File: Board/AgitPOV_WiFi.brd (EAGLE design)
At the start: 41.5 x 67.6 mm, 45 parts, among them U1 MMA8452Q

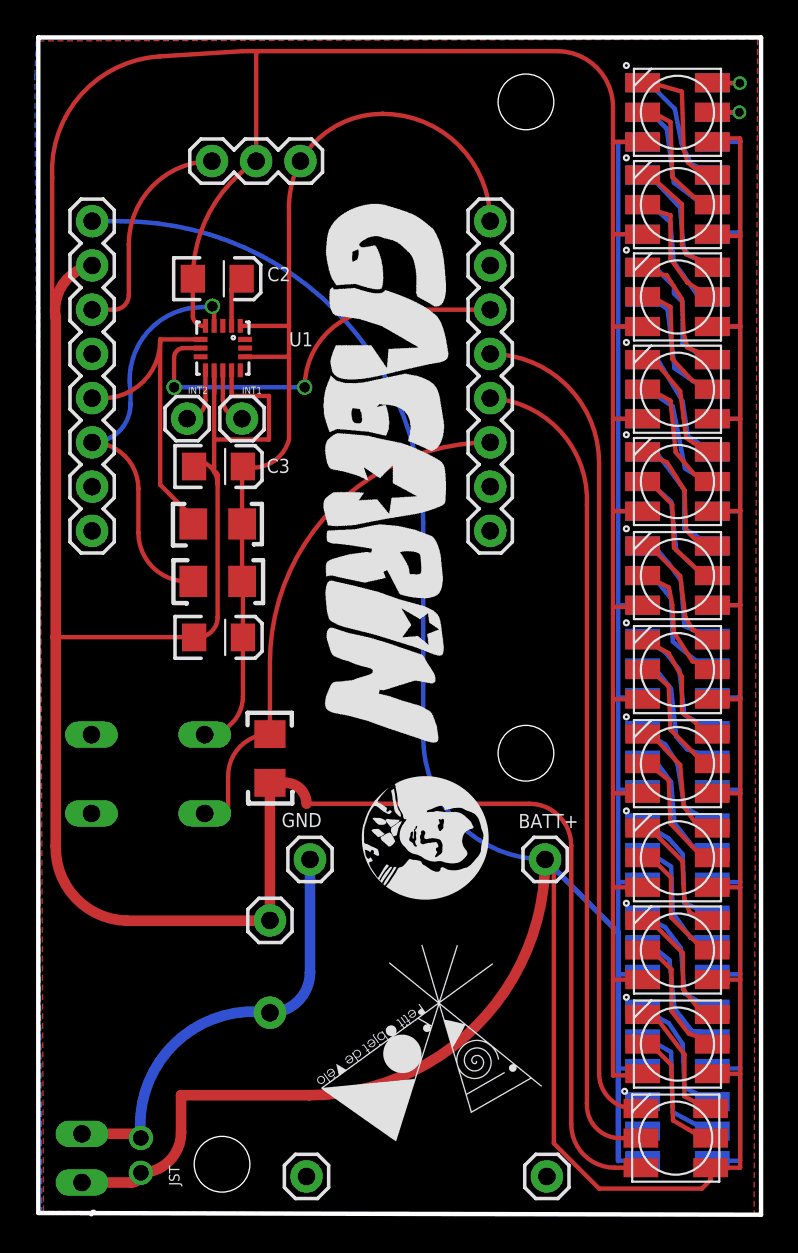
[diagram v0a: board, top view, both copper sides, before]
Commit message: Mean and lean board
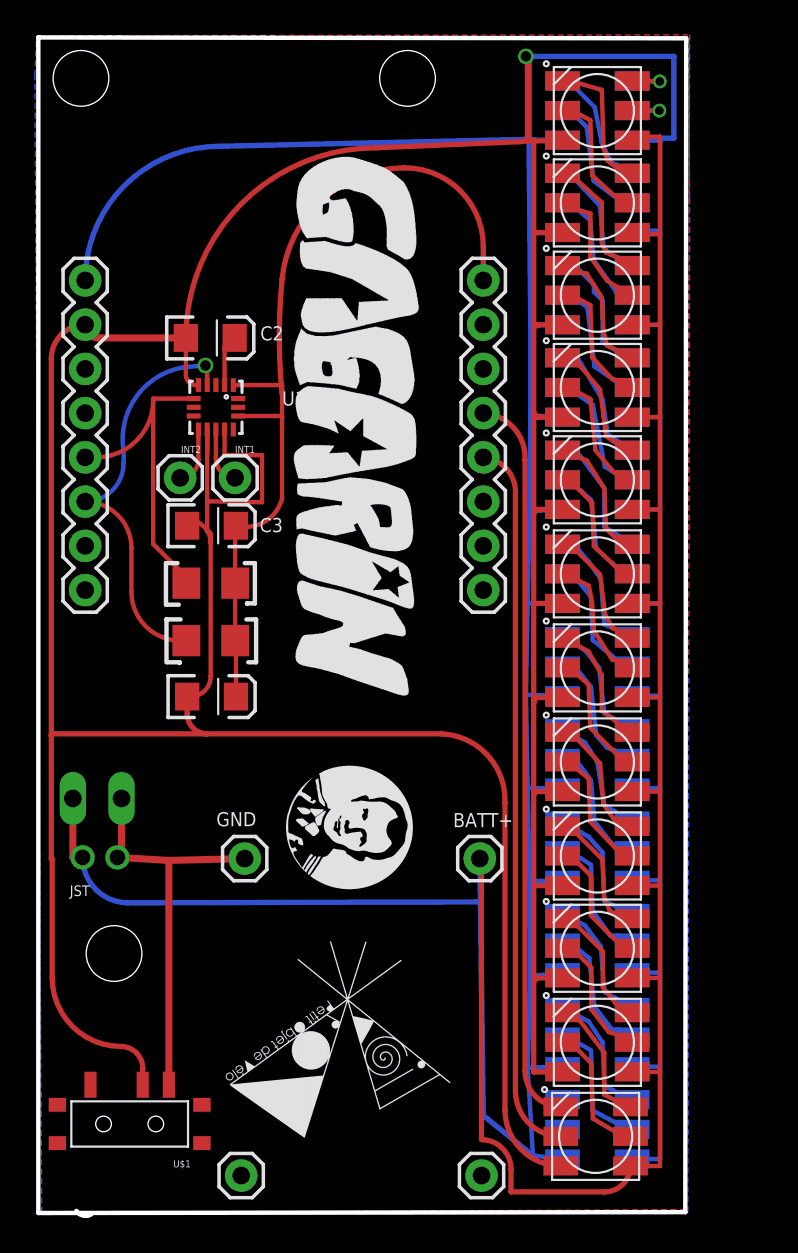
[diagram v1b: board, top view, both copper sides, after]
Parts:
- removed HALL: Hall, SparkFun-Connectors:1X03
- removed JP-GND: SWITCH, SparkFun-Connectors:1X01
- removed JP-GNDE: -, SparkFun-Connectors:1X01
- removed PUSHBUTTON: (no value), switch-omron:B3F-10XX
- removed R3: 10k, SparkFun-Resistors:1206
- added U$1: SWITCH_SPDT, SparkFun-Electromechanical:KPS-1290
- moved BATT 19.5 mm to (5.01, 24.1), turned to 0 degrees
- moved JST 17.3 mm to (3.90, 20.8), turned to 270 degrees
- moved DEL1 4.60 mm to (32.4, 4.74)
- moved DEL10 4.60 mm to (32.5, 53.0)
- moved DEL11 4.60 mm to (32.5, 58.3)
- moved DEL12 4.60 mm to (32.5, 63.6)
- moved DEL13 4.60 mm to (32.5, 63.6)
- moved DEL15 4.60 mm to (32.5, 53.0)
- moved DEL17 4.60 mm to (32.5, 42.4)
- moved DEL18 4.60 mm to (32.5, 37.0)
- moved DEL19 4.60 mm to (32.5, 31.7)
- moved DEL2 4.60 mm to (32.5, 10.1)
- moved DEL20 4.60 mm to (32.5, 26.4)
- moved DEL21 4.60 mm to (32.5, 21.1)
- moved DEL22 4.60 mm to (32.5, 15.8)
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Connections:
- removed net PULLDOWN: PUSHBUTTON.3, R3.2, WEMOS1.3
- removed net SA0: U1.7, WEMOS1.6
- net +3.3V: no longer HALL.1, PUSHBUTTON.1
- net ENTREEGND: now also U$1.S; no longer JP-GNDE.1
- net GND: now also U$1.P; no longer HALL.2, JP-GND.1, R3.1
- net N$41: no longer HALL.3
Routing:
- net PULLDOWN: track 28.9 -> 0.00 mm
- net SA0: track 23.5 -> 0.00 mm, vias 2 -> 0
- net 5V: track 284.5 -> 262.4 mm
- net GND: track 348.7 -> 332.9 mm, vias 0 -> 1
- net N$41: track 12.1 -> 0.00 mm
- net N$2: track 46.6 -> 40.8 mm
- net +3.3V: track 55.0 -> 49.2 mm
- net N$4: track 47.1 -> 41.6 mm
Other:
- board size 41.5 x 67.6 mm -> 37.2 x 67.7 mm
- board text removed: "D0"
- board text removed: "D8"
- board text removed: "R1"
